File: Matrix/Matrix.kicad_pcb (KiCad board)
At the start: 2 copper layers, 120.1 x 106.4 mm, 169 parts, among them J1 Conn_01x08, J2 USB_C_Receptacle_USB2.0_16P, Q1 2N2219, Q10 2N2219, Q11 2N2219, Q12 2N2219, Q13 2N2219, Q14 2N2219, Q15 2N2219, Q16 2N2219, Q2 2N2219, Q3 2N2219, Q4 2N2219, Q5 2N2219, Q6 2N2219, Q7 2N2219, Q8 2N2219, Q9 2N2219, U1 74HC138, U10 ESP32-S3, U11 AP2112K-3.3, U12 ER_OLEDM0.91_1x-I2C, U13 W25Q32JVSS, U2 74HC574N, U3 74HC574N, U4 74HC574N, U5 74HC574N, U6 74HC574N, U7 74HC574N, U8 74HC574N, U9 74HC574N, Y1 40MHz (+-10ppm)

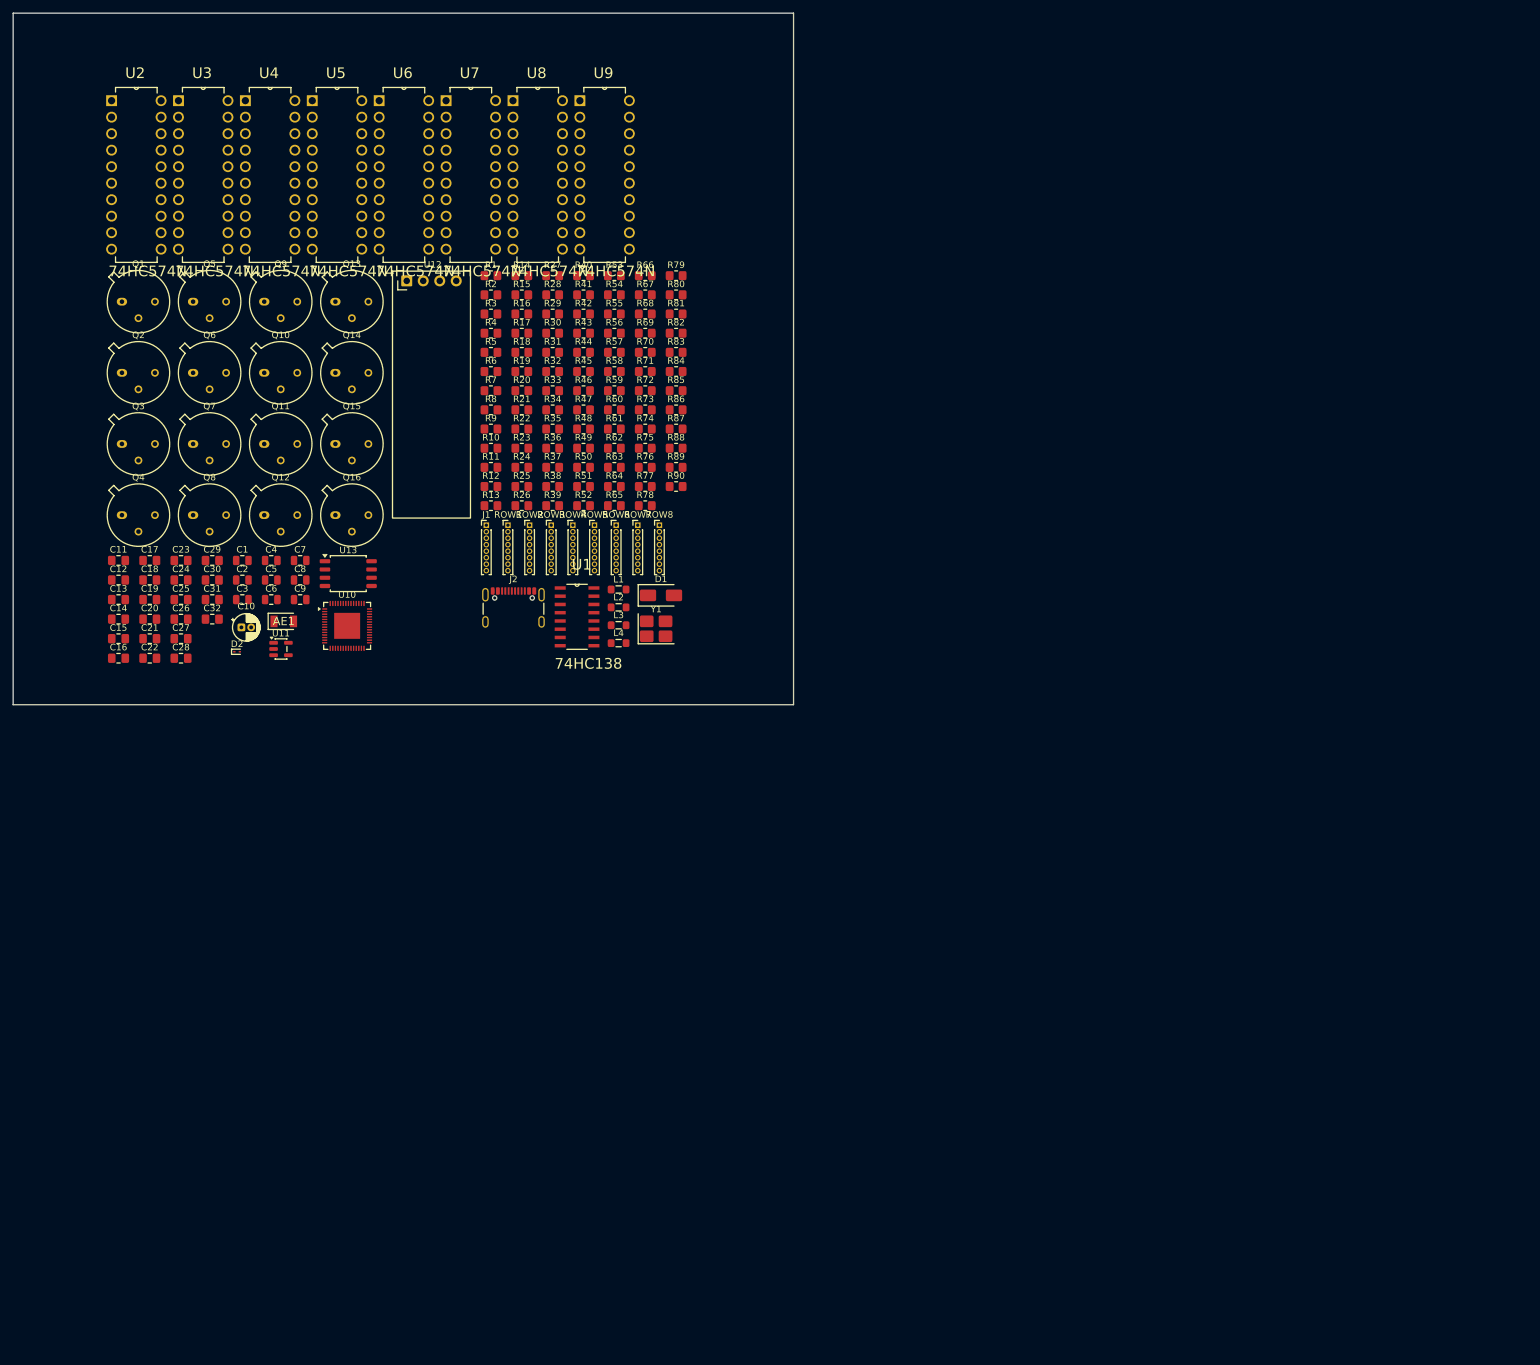
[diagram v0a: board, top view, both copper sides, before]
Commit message: Update Matrix.kicad_pcb
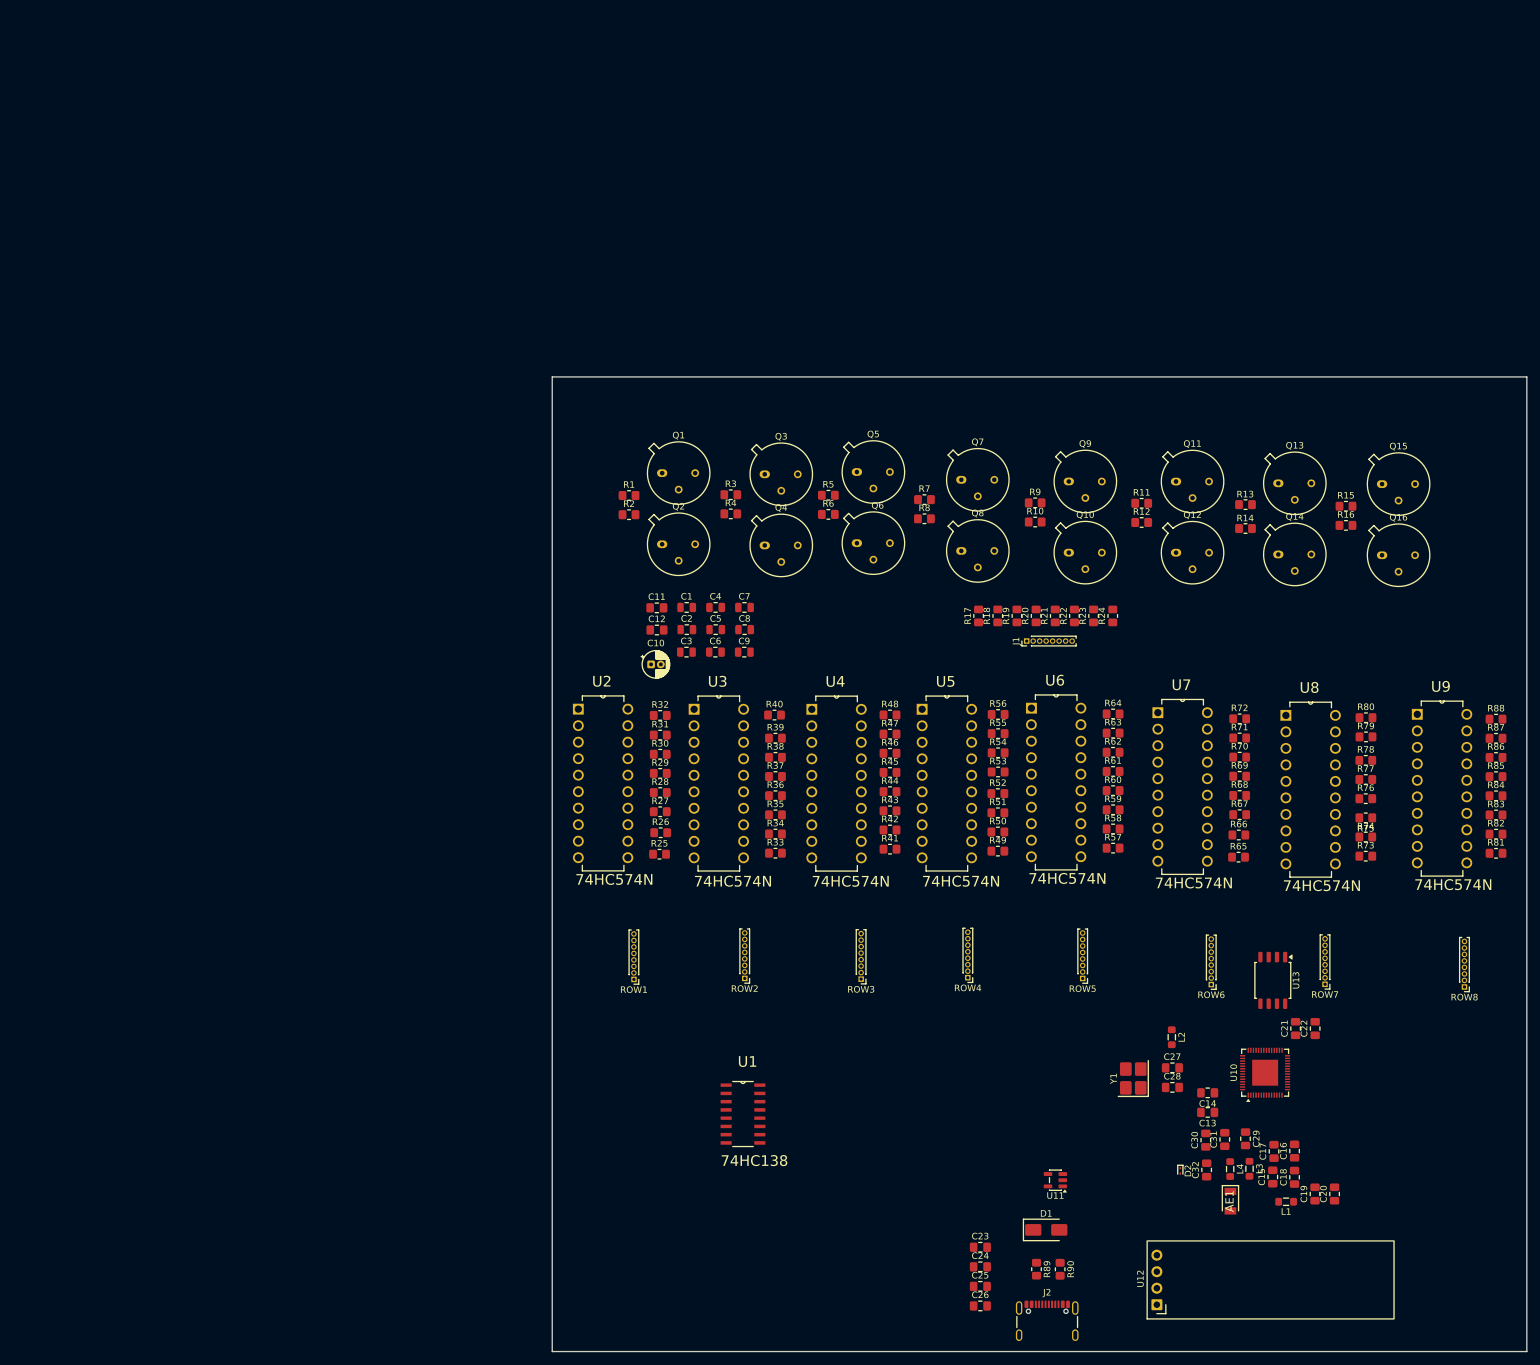
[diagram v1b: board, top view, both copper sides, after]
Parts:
- moved C20 202.7 mm to (294.2, 229.3), turned to 90 degrees
- moved C19 201.3 mm to (291.2, 229.3), turned to 90 degrees
- moved C18 198.7 mm to (288.1, 226.7), turned to 90 degrees
- moved C16 196.3 mm to (288.1, 222.7), turned to 90 degrees
- moved C15 196.0 mm to (284.7, 226.6), turned to 90 degrees
- moved C17 195.5 mm to (284.9, 222.7), turned to 90 degrees
- moved U12 195.3 mm to (266.9, 246.3), turned to 90 degrees
- moved C22 188.2 mm to (291.2, 203.8), turned to 90 degrees
- moved C21 186.3 mm to (288.2, 203.8), turned to 90 degrees
- moved C13 185.3 mm to (274.7, 216.7), turned to 180 degrees
- moved C14 182.8 mm to (274.7, 213.7), turned to 180 degrees
- moved C29 182.2 mm to (280.5, 220.8), turned to -90 degrees
- moved C31 176.6 mm to (277.3, 220.9), turned to 90 degrees
- moved C30 175.5 mm to (274.4, 221.0), turned to 90 degrees
- moved C32 175.0 mm to (274.5, 225.6), turned to 90 degrees
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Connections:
- C1 pad 1: +5V -> +3.3V
- C2 pad 1: +5V -> +3.3V
- C3 pad 1: +5V -> +3.3V
- C4 pad 1: +5V -> +3.3V
- C5 pad 1: +5V -> +3.3V
- C6 pad 1: +5V -> +3.3V
- C7 pad 1: +5V -> +3.3V
- C8 pad 1: +5V -> +3.3V
- C9 pad 1: +5V -> +3.3V
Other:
- board size 120.1 x 106.4 mm -> 150 x 150 mm
